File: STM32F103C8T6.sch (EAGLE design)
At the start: 38 parts, among them J3 AVX_009159010061916AVX_009159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, J4 CORTEX_DEBUG_PTH, J6 455-1750-1-ND, J7 455-1750-1-ND, U1 STM32F103C8T6, U2 CJT1117-3.3-SOT223

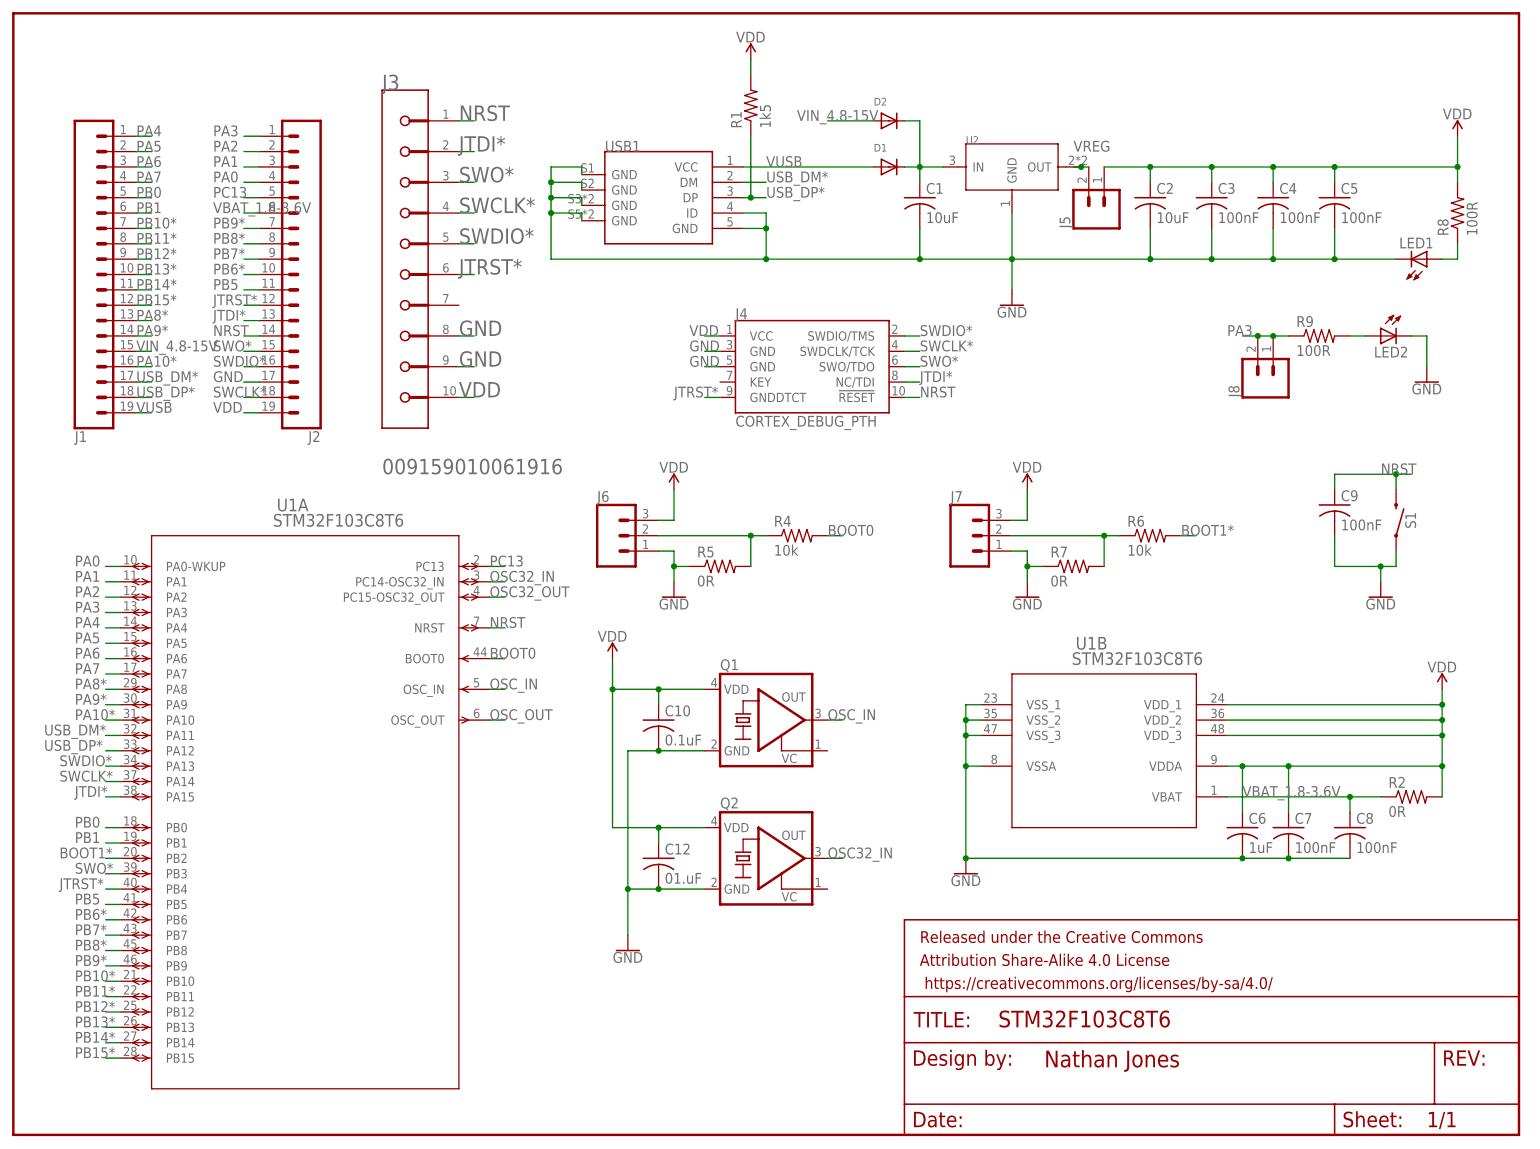
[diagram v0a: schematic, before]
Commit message: Finished layout.
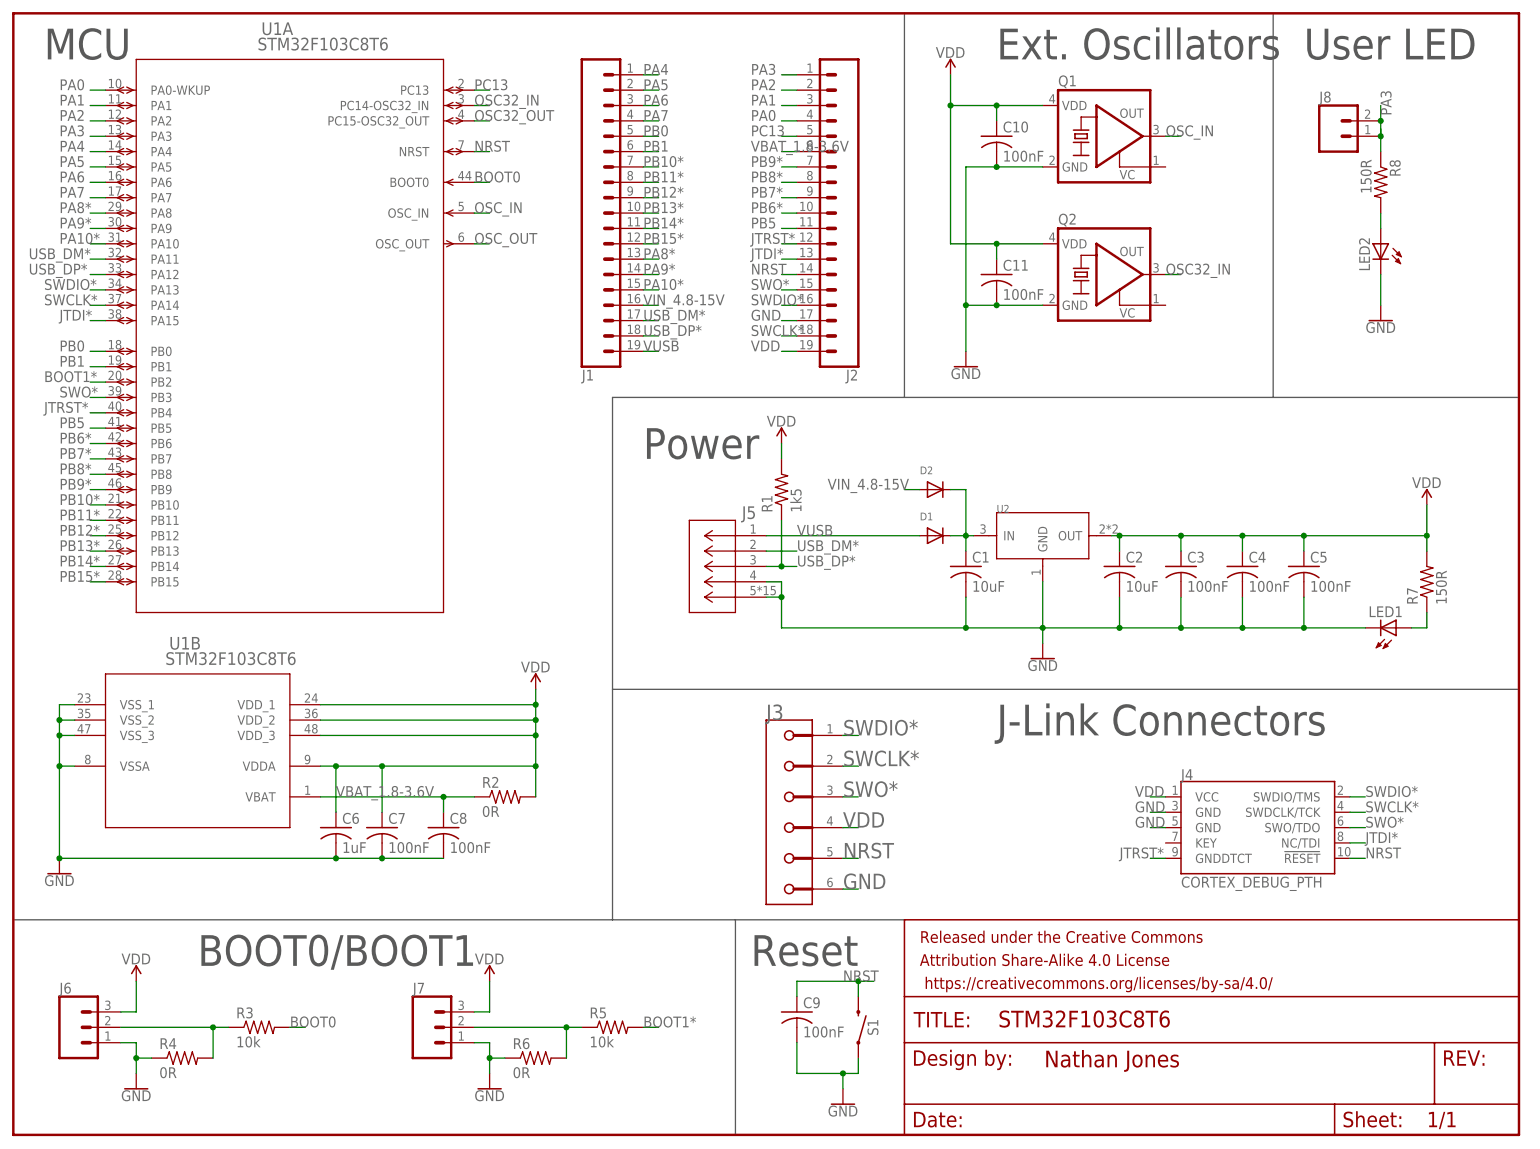
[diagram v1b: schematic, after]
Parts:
- removed C12: 01.uF, adafruit:C-USC0402
- removed R9: 100R, adafruit:R-US_R0402
- removed USB1: 10118193-0001LF, OPL_Connector:MICRO-USB-SMD-B-(10118193-0001LF)
- added C11: 100nF, adafruit:C-USC0402
- added R3: 10k, adafruit:R-US_R0402
- C1, C2: LCSC_PART (none) -> C15525
- C10: value 0.1uF -> 100nF; LCSC_PART (none) -> C1525
- C3, C4, C5, C7, C8, C9: LCSC_PART (none) -> C1525
- C6: LCSC_PART (none) -> C52923
- D1, D2: LCSC_PART (none) -> C8598
- J3: value AVX_009159010061916AVX_009159010061916_0_0 -> AVX_6-PIN_009159006061916; device AVX - 009159010061916:AVX_009159010061916AVX_009159010061916_0_0 -> Debug-Edge_AVX-connectors:AVX_6-PIN_009159006061916
- J5: value (none) -> 10118194-0001LF; device SparkFun-Connectors:CONN_02 -> USB-micro-B_Amphenol_10118194-0001LF:10118194-0001LF
- J6, J7: value 455-1750-1-ND -> (none); device SparkFun-Connectors:CONN_03 -> SparkFun-Connectors:CONN_031X03_NO_SILK
- J8: device SparkFun-Connectors:CONN_02 -> SparkFun-Connectors:CONN_021X02_NO_SILK
- LED1: LCSC_PART (none) -> C72041
- LED2: LCSC_PART (none) -> C72038
- R1: LCSC_PART (none) -> C25867
- R2: LCSC_PART (none) -> C17168
- R4, R6: value 10k -> 0R; LCSC_PART (none) -> C17168
- R5: value 0R -> 10k; LCSC_PART (none) -> C25744
- R7: value 0R -> 150R; LCSC_PART (none) -> C25082
- R8: value 100R -> 150R; LCSC_PART (none) -> C25082
- S1: LCSC_PART (none) -> C318884
- U1: LCSC_PART (none) -> C94046
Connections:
- removed net VREG: J5.2, U2.OUT
- net BOOT0: now also R3.2; no longer R4.2
- net BOOT1*: now also R5.2; no longer R6.2
- net GND: now also C11.2, J3.6, J5.4, J5.5, R4.1, R6.1; no longer C12.2, J3.8, J3.9, R5.1, R7.1, USB1.GND@1, USB1.GND@2, USB1.GND@3, USB1.GND@4, USB1.GND@5, USB1.ID
- net JTDI*: no longer J3.2
- net JTRST*: no longer J3.6
- net N$1: now also R3.1, R4.2; no longer R4.1, R5.2
- net N$4: now also R8.2; no longer R9.2
- net N$6: now also R5.1, R6.2; no longer R6.1, R7.2
- net N$7: now also R7.1; no longer R8.1
- net NRST: now also J3.5; no longer J3.1
- net PA10*: now also J1.15; no longer J1.16
- net PA3: now also R8.1; no longer R9.1
- net SWCLK*: now also J3.2; no longer J3.4
- net SWDIO*: now also J3.1; no longer J3.5
- net USB_DM*: now also J5.2; no longer USB1.DM
- net USB_DP*: now also J5.3; no longer USB1.DP
- net VDD: now also C11.1, J3.4, R7.2, U2.OUT; no longer C12.1, J3.10, J5.1, R8.2
- net VIN_4.8-15V: now also J1.16; no longer J1.15
- net VUSB: now also J5.1; no longer USB1.VCC
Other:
- note added: "BOOT0/BOOT1"
- note added: "Ext. Oscillators"
- note added: "J-Link Connectors"
- note added: "MCU"
- note added: "Power"
- note added: "Reset"
- note added: "User LED"
- moved on the sheet: C1, C10, C2, C3, C4, C5, C6, C7, C8, C9, D1, D2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
